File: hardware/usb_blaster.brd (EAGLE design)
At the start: 58.3 x 15.2 mm, 18 parts, among them IC2 PIC18F14K50SO, X1 53047-06

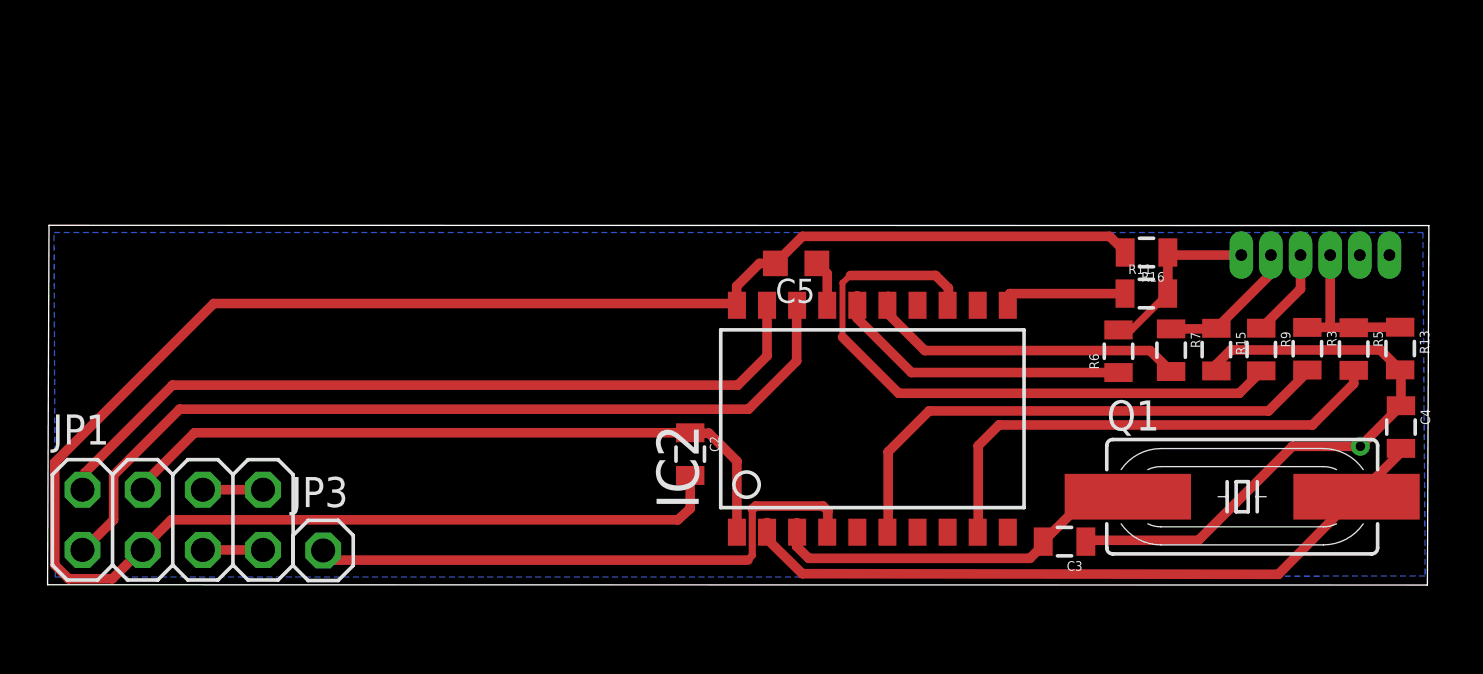
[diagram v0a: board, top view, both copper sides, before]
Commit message: Añado splitter
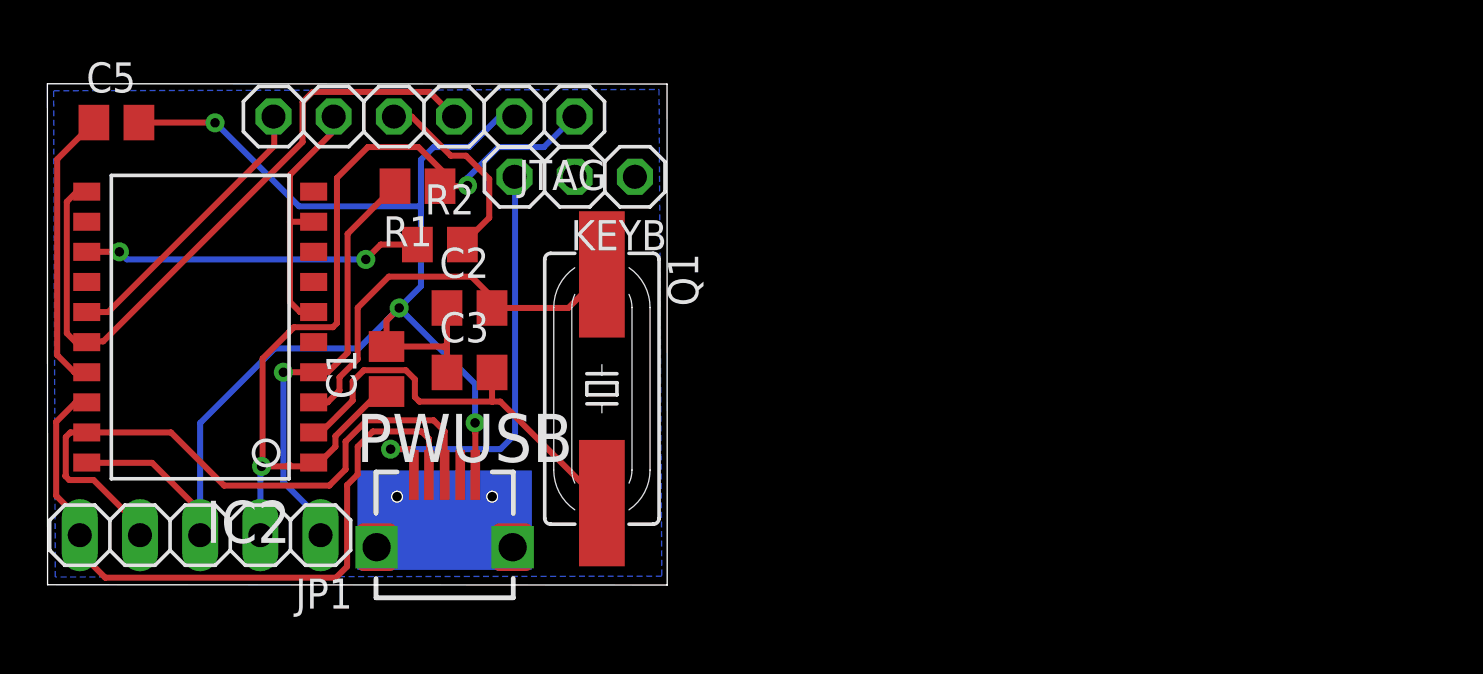
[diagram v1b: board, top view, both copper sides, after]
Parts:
- removed C4: 22p, SparkFun:0805
- removed JP3: (no value), pinhead:1X01
- removed R11, R3, R5, R6, R7, R9: 100R, SparkFun:0805
- removed R13, R15, R16: 220R, SparkFun:0805
- removed X1: 53047-06, con-molex:53047-06
- added C1: 4.7u, rcl:C0805
- added JTAG: (no value), pinhead:1X06
- added KEYB: (no value), pinhead:1X03
- added PWUSB: MICROUSB, zxuno_rev_mcleod:MICRO_USB_1PRIMARY
- added R1: 10K, rcl:R0805
- added R2: 100R, rcl:R0805
- C2: value 4.7u -> 22p; device SparkFun:0805 -> rcl:C0805
- C3: device SparkFun:0805 -> rcl:C0805
- C5: device rcl:C0603K -> rcl:C0805
- JP1: device pinhead:2X04 -> pinhead:1X05
- moved C5 29.3 mm to (2.90, 19.5), turned to 0 degrees
- moved IC2 27.9 mm to (6.44, 10.2), turned to 90 degrees
- moved Q1 27.4 mm to (23.4, 8.27), turned to 270 degrees
- moved C3 26.1 mm to (17.8, 8.96), turned to 0 degrees
- moved C2 11.2 mm to (17.8, 11.7), turned to 0 degrees
- moved JP1 1.33 mm to (6.44, 2.09), turned to 180 degrees
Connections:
- removed net N$13: IC2.9, R5.2
- removed net N$16: IC2.11, R11.1
- removed net N$2: IC2.15, R7.2
- removed net N$3: JP1.6, JP1.8
- removed net N$5: JP1.5, JP1.7
- removed net N$6: IC2.16, R6.1
- removed net N$8: IC2.6, R3.2
- new net 3.3V: C1.1, IC2.1, JP1.2, JTAG.1, R1.1
- new net CLKPS2: KEYB.1
- new net DATAPS2: KEYB.2
- net GND: now also C1.2, C2.1, JTAG.2, PWUSB.5; no longer C2.2, C4.1, R13.2, R15.2, R16.2, X1.5
- net N$1: now also C3.2; no longer C4.2
- net N$4: now also C2.2; no longer C3.2
- net N$7: now also R2.1; no longer R9.2
- net PGC: now also JP1.5, PWUSB.2; no longer JP1.1
- net PGD: now also JP1.4, PWUSB.3; no longer JP1.2
- net TCK: now also IC2.11, IC2.16, JTAG.3; no longer R11.2, R16.1, R6.2, X1.1
- net TDI: now also IC2.6, IC2.9, JTAG.5; no longer R13.1, R3.1, R5.1, X1.4
- net TDO: now also JTAG.4, R2.2; no longer R9.1, X1.3
- net TMS: now also IC2.15, JTAG.6; no longer R15.1, R7.1, X1.2
- net VCC: now also KEYB.3, PWUSB.1; no longer C2.1, IC2.1, JP1.4
- net VPP: now also JP1.1, R1.2; no longer JP3.1
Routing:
- net GND: track 109.8 -> 62.0 mm, vias 1 -> 3
- net 3.3V: track 0.00 -> 37.3 mm, vias 0 -> 2
- net N$8: track 22.6 -> 0.00 mm
- net TCK: track 7.59 -> 28.9 mm
- net N$13: track 21.1 -> 0.00 mm
- net N$2: track 14.1 -> 0.00 mm
- net N$6: track 13.3 -> 0.00 mm
- net N$1: track 30.8 -> 17.7 mm
- net N$7: track 26.9 -> 14.4 mm, vias 0 -> 2
- net VCC: track 29.7 -> 18.4 mm, vias 0 -> 1
- net N$12: track 1.95 -> 12.0 mm
- net PGC: track 36.9 -> 29.6 mm
- net PGD: track 33.7 -> 26.9 mm
- net VPP: track 24.6 -> 18.4 mm, vias 0 -> 1
- net TMS: track 5.96 -> 12.1 mm
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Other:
- board size 58.3 x 15.2 mm -> 26.2 x 21.2 mm
